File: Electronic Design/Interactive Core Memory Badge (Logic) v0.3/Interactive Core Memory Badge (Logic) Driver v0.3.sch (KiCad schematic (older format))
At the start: 64 parts, among them J1 SSW-116-22-F-S-VS‎, J2 SSW-116-22-F-S-VS‎, Q10 MMBT4401LT1G, Q11 MMBT4403LT1G, Q12 MMBT4401LT1G, Q13 MMBT4403LT1G, Q14 MMBT4401LT1G, Q15 MMBT4403LT1G, Q16 MMBT4401LT1G, Q17 MMBT4403LT1G, Q18 MMBT4401LT1G, Q19 MMBT4403LT1G, Q2 MMBT4403LT1G, Q20 MMBT4401LT1G, Q21 MMBT4403LT1G, Q22 MMBT4401LT1G, Q3 MMBT4401LT1G, Q4 MMBT4401LT1G, Q5 MMBT4403LT1G, Q6 MMBT4401LT1G, Q7 MMBT4403LT1G, Q8 MMBT4401LT1G, Q9 MMBT4403LT1G

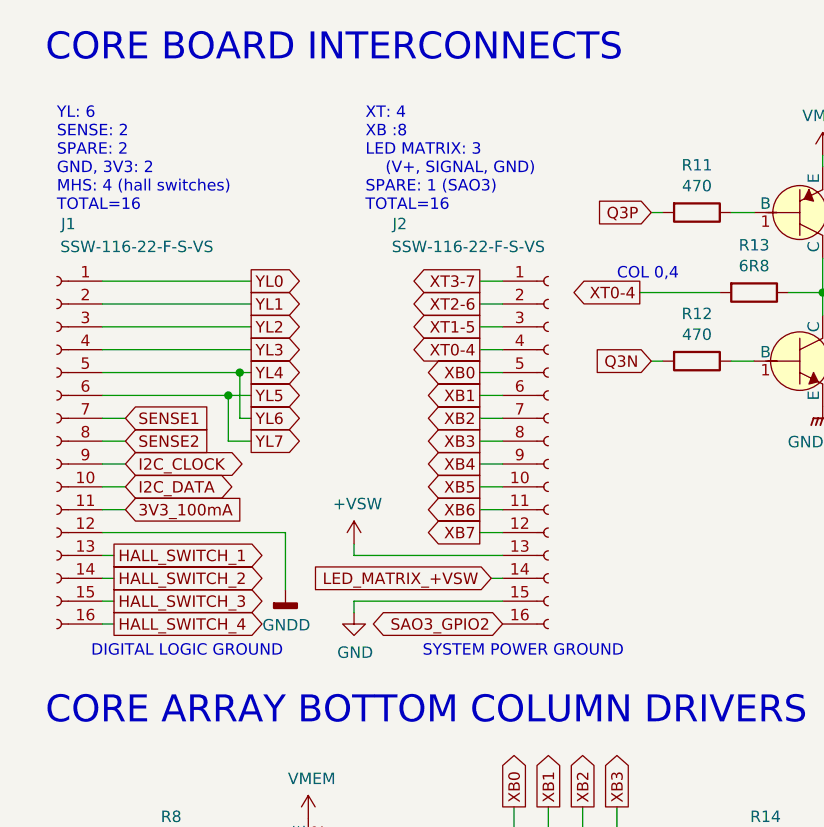
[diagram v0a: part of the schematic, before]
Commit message: Schematic review tweaks
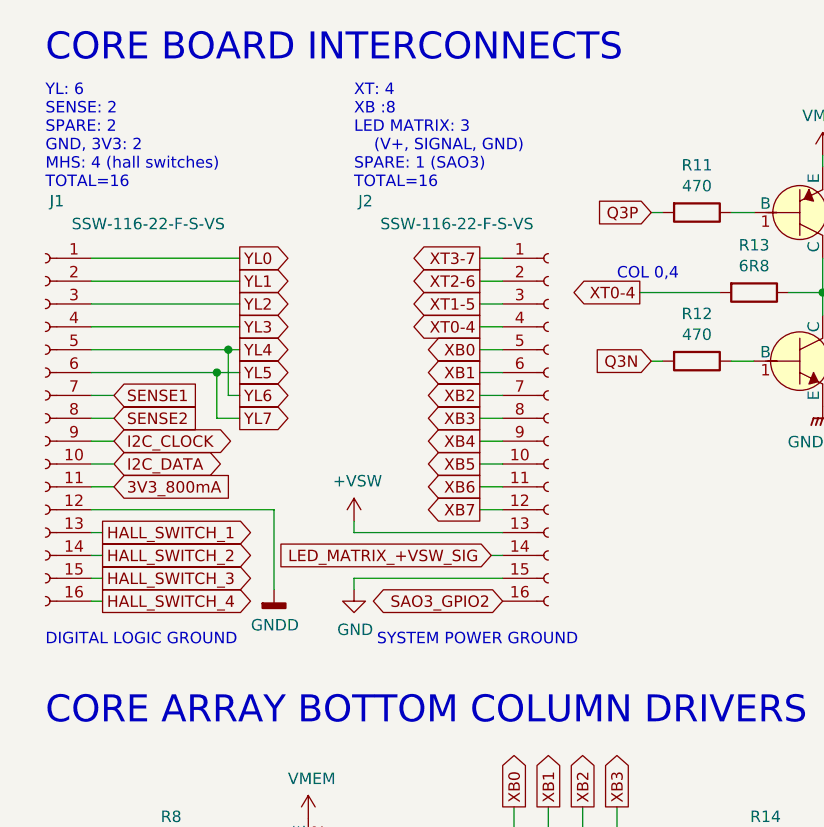
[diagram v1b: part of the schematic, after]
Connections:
- net 3V3_100mA is gone; now on net VMEM: J1.11 (Pin_11)
- net LED_MATRIX_+VSW renamed LED_MATRIX_+VSW_SIG
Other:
- moved on the sheet: J1, J2
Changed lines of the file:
@@
 Wire Wire Line
 	1200 4450 2400 4450
+Text GLabel 2450 2300 0    50   Output ~ 0
+XB3
+Text GLabel 2450 2200 0    50   Output ~ 0
+XB2
+Text GLabel 2450 2100 0    50   Output ~ 0
+XB1
+Text GLabel 2450 2000 0    50   Output ~ 0
+XB0
 Text GLabel 2450 2400 0    50   Output ~ 0
-XB3
-Text GLabel 2450 2300 0    50   Output ~ 0
-XB2
-Text GLabel 2450 2200 0    50   Output ~ 0
-XB1
-Text GLabel 2450 2100 0    50   Output ~ 0
-XB0
+XB4
 Text GLabel 2450 2500 0    50   Output ~ 0
-XB4
+XB5
 Text GLabel 2450 2600 0    50   Output ~ 0
-XB5
+XB6
 Text GLabel 2450 2700 0    50   Output ~ 0
-XB6
-Text GLabel 2450 2800 0    50   Output ~ 0
 XB7
-Text GLabel 2450 2000 0    50   Output ~ 0
+Text GLabel 2450 1900 0    50   Output ~ 0
 XT0-4
-Text GLabel 2450 1900 0    50   Output ~ 0
+Text GLabel 2450 1800 0    50   Output ~ 0
 XT1-5
-Text GLabel 2450 1800 0    50   Output ~ 0
+Text GLabel 2450 1700 0    50   Output ~ 0
 XT2-6
-Text GLabel 2450 1700 0    50   Output ~ 0
+Text GLabel 2450 1600 0    50   Output ~ 0
 XT3-7
 Wire Wire Line
+	2450 1600 2550 1600
+Wire Wire Line
 	2450 1700 2550 1700
 Wire Wire Line
@@
 Wire Wire Line
 	2450 1900 2550 1900
-Wire Wire Line
-	2450 2000 2550 2000
-Text GLabel 1450 1800 2    50   Output ~ 0
+Text GLabel 1400 1700 2    50   Output ~ 0
 YL1
-Text GLabel 1450 1700 2    50   Output ~ 0
+Text GLabel 1400 1600 2    50   Output ~ 0
 YL0
-Text GLabel 1450 1900 2    50   Output ~ 0
+Text GLabel 1400 1800 2    50   Output ~ 0
 YL2
-Text GLabel 1450 2000 2    50   Output ~ 0
+Text GLabel 1400 1900 2    50   Output ~ 0
 YL3
-Text GLabel 1450 2400 2    50   Output ~ 0
+Text GLabel 1400 2300 2    50   Output ~ 0
 YL7
 Wire Wire Line
-	1400 2100 1400 2300
-Wire Wire Line
-	1400 2300 1450 2300
-Wire Wire Line
-	1450 1700 800  1700
-Wire Wire Line
-	1450 2000 800  2000
-Wire Wire Line
-	1450 2100 1400 2100
-Wire Wire Line
-	1400 2100 800  2100
-Connection ~ 1400 2100
-Wire Wire Line
-	1350 2400 1450 2400
-Wire Wire Line
-	1350 2200 1350 2400
-Wire Wire Line
-	1450 2200 1350 2200
-Text Notes 600  1400 0    50   ~ 0
+	1350 2000 1350 2200
+Wire Wire Line
+	1350 2200 1400 2200
+Wire Wire Line
+	1400 1600 750  1600
+Wire Wire Line
+	1400 1900 750  1900
+Wire Wire Line
+	1400 2000 1350 2000
+Wire Wire Line
+	1350 2000 750  2000
+Connection ~ 1350 2000
+Wire Wire Line
+	1300 2300 1400 2300
+Wire Wire Line
+	1300 2100 1300 2300
+Wire Wire Line
+	1400 2100 1300 2100
+Text Notes 550  1300 0    50   ~ 0
 YL: 6\nSENSE: 2\nSPARE: 2\nGND, 3V3: 2\nMHS: 4 (hall switches)\nTOTAL=16
 Wire Wire Line
-	1350 2200 800  2200
-Connection ~ 1350 2200
-Wire Wire Line
-	2450 2800 2550 2800
+	1300 2100 750  2100
+Connection ~ 1300 2100
 Wire Wire Line
 	2450 2700 2550 2700
+Wire Wire Line
+	2450 2600 2550 2600
 $Comp
 L Connector:Conn_01x16_Female J2
 U 1 1 5E78B5ED
-P 2750 2400
-F 0 "J2" H 2100 3350 50  0000 C CNN
-F 1 "SSW-116-22-F-S-VS‎" H 2400 3250 50  0000 C CNN
-F 2 "Connector_PinHeader_2.54mm:PinHeader_1x16_P2.54mm_Vertical_SMD_and_TH_Pin1Left" H 2750 2400 50  0001 C CNN
-F 3 "~" H 2750 2400 50  0001 C CNN
-	1    2750 2400
+P 2750 2300
+F 0 "J2" H 1950 3250 50  0000 C CNN
+F 1 "SSW-116-22-F-S-VS‎" H 2350 3150 50  0000 C CNN
+F 2 "Connector_PinHeader_2.54mm:PinHeader_1x16_P2.54mm_Vertical_SMD_and_TH_Pin1Left" H 2750 2300 50  0001 C CNN
+F 3 "~" H 2750 2300 50  0001 C CNN
+	1    2750 2300
 	1    0    0    -1
 $EndComp
@@
 L Connector:Conn_01x16_Female J1
 U 1 1 5E78B5F3
-P 600 2400
-F 0 "J1" H 550 3350 50  0000 C CNN
-F 1 "SSW-116-22-F-S-VS‎" H 250 3250 50  0000 C CNN
-F 2 "Connector_PinHeader_2.54mm:PinHeader_1x16_P2.54mm_Vertical_SMD_and_TH_Pin1Left" H 600 2400 50  0001 C CNN
-F 3 "~" H 600 2400 50  0001 C CNN
-	1    600  2400
+P 550 2300
+F 0 "J1" H 500 3250 50  0000 C CNN
+F 1 "SSW-116-22-F-S-VS‎" H 100 3150 50  0000 C CNN
+F 2 "Connector_PinHeader_2.54mm:PinHeader_1x16_P2.54mm_Vertical_SMD_and_TH_Pin1Left" H 550 2300 50  0001 C CNN
+F 3 "~" H 550 2300 50  0001 C CNN
+	1    550  2300
 	-1   0    0    -1
 $EndComp
-Text Notes 1950 1400 0    50   ~ 0
+Text Notes 1900 1300 0    50   ~ 0
 XT: 4\nXB :8\nLED MATRIX: 3\n    (V+, SIGNAL, GND)\nSPARE: 1 (SAO3)\nTOTAL=16
 Wire Wire Line
-	2450 2400 2550 2400
-Wire Wire Line
-	2450 2600 2550 2600
-Text GLabel 900  2300 2    50   Input ~ 0
+	2450 2300 2550 2300
+Wire Wire Line
+	2450 2500 2550 2500
+Text GLabel 850  2200 2    50   Input ~ 0
 SENSE1
-Text GLabel 900  2400 2    50   Input ~ 0
+Text GLabel 850  2300 2    50   Input ~ 0
 SENSE2
 Wire Wire Line
-	900  2400 800  2400
-Text GLabel 2500 3000 0    50   Input ~ 0
-LED_MATRIX_+VSW
-Wire Wire Line
-	2500 3000 2550 3000
+	850  2300 750  2300
+Text GLabel 2500 2900 0    50   Input ~ 0
+LED_MATRIX_+VSW_SIG
+Wire Wire Line
+	2500 2900 2550 2900
 $Comp
 L power:GNDD #PWR0164
 U 1 1 5E78B651
-P 1600 3050
-F 0 "#PWR0164" H 1600 2800 50  0001 C CNN
-F 1 "GNDD" H 1604 2895 50  0000 C CNN
-F 2 "" H 1600 3050 50  0001 C CNN
-F 3 "" H 1600 3050 50  0001 C CNN
-	1    1600 3050
-	1    0    0    -1
-$EndComp
-Text GLabel 850  2900 2    50   Output ~ 0
+P 1550 3050
+F 0 "#PWR0164" H 1550 2800 50  0001 C CNN
+F 1 "GNDD" H 1554 2895 50  0000 C CNN
+F 2 "" H 1550 3050 50  0001 C CNN
+F 3 "" H 1550 3050 50  0001 C CNN
+	1    1550 3050
+	1    0    0    -1
+$EndComp
+Text GLabel 800  2800 2    50   Output ~ 0
 HALL_SWITCH_1
-Text GLabel 850  3000 2    50   Output ~ 0
+Text GLabel 800  2900 2    50   Output ~ 0
 HALL_SWITCH_2
-Text GLabel 850  3100 2    50   Output ~ 0
+Text GLabel 800  3000 2    50   Output ~ 0
 HALL_SWITCH_3
-Text GLabel 850  3200 2    50   Output ~ 0
+Text GLabel 800  3100 2    50   Output ~ 0
 HALL_SWITCH_4
 Wire Wire Line
-	1600 2800 1600 3050
-Wire Wire Line
-	800  2700 900  2700
-Wire Wire Line
-	800  2800 1600 2800
-Wire Wire Line
-	850  3000 800  3000
-Wire Wire Line
-	850  3200 800  3200
+	1550 2700 1550 3050
+Wire Wire Line
+	750  2600 850  2600
+Wire Wire Line
+	750  2700 1550 2700
+Wire Wire Line
+	800  2900 750  2900
+Wire Wire Line
+	800  3100 750  3100
+Wire Wire Line
+	2550 2000 2450 2000
 Wire Wire Line
 	2550 2100 2450 2100
@@
 	2550 2200 2450 2200
 Wire Wire Line
-	2550 2300 2450 2300
-Wire Wire Line
-	2550 2500 2450 2500
-Wire Wire Line
-	2550 3100 1900 3100
-Text Notes 750  3350 0    50   ~ 0
+	2550 2400 2450 2400
+Wire Wire Line
+	2550 3000 1900 3000
+Text Notes 550  3300 0    50   ~ 0
 DIGITAL LOGIC GROUND
 Text Notes 4200 7750 0    50   ~ 0
@@
 L power:GND #PWR?
 U 1 1 5E79F49F
-P 1900 3150
+P 1900 3050
 AR Path="/5D254AE8/5E79F49F" Ref="#PWR?"  Part="1"
 AR Path="/5E79F49F" Ref="#PWR?"  Part="1"
 AR Path="/5E755AC8/5E79F49F" Ref="#PWR0165"  Part="1"
-F 0 "#PWR0165" H 1900 2900 50  0001 C CNN
-F 1 "GND" H 1905 2975 50  0000 C CNN
-F 2 "" H 1900 3150 50  0001 C CNN
-F 3 "" H 1900 3150 50  0001 C CNN
-	1    1900 3150
-	1    0    0    -1
-$EndComp
-Text GLabel 900  2700 2    50   Input ~ 0
-3V3_100mA
-Wire Wire Line
-	800  1800 1450 1800
-Wire Wire Line
-	800  1900 1450 1900
-Wire Wire Line
-	800  2300 900  2300
-Wire Wire Line
-	800  2900 850  2900
-Wire Wire Line
-	800  3100 850  3100
-Text Notes 2200 3350 0    50   ~ 0
+F 0 "#PWR0165" H 1900 2800 50  0001 C CNN
+F 1 "GND" H 1905 2875 50  0000 C CNN
+F 2 "" H 1900 3050 50  0001 C CNN
+F 3 "" H 1900 3050 50  0001 C CNN
+	1    1900 3050
+	1    0    0    -1
+$EndComp
+Text GLabel 850  2600 2    50   Input ~ 0
+3V3_800mA
+Wire Wire Line
+	750  1700 1400 1700
+Wire Wire Line
+	750  1800 1400 1800
+Wire Wire Line
+	750  2200 850  2200
+Wire Wire Line
+	750  2800 800  2800
+Wire Wire Line
+	750  3000 800  3000
+Text Notes 2000 3300 0    50   ~ 0
 SYSTEM POWER GROUND
 Text Notes 550  750  0    118  ~ 0
@@
 L power:+VSW #PWR0122
 U 1 1 5E76A192
-P 1900 2850
-F 0 "#PWR0122" H 1900 2700 50  0001 C CNN
-F 1 "+VSW" H 1915 3025 50  0000 C CNN
-F 2 "" H 1900 2850 50  0001 C CNN
-F 3 "" H 1900 2850 50  0001 C CNN
-	1    1900 2850
-	1    0    0    -1
-$EndComp
-Wire Wire Line
-	1900 2900 1900 2850
-Wire Wire Line
-	1900 2900 2550 2900
+P 1900 2750
+F 0 "#PWR0122" H 1900 2600 50  0001 C CNN
+F 1 "+VSW" H 1915 2925 50  0000 C CNN
+F 2 "" H 1900 2750 50  0001 C CNN
+F 3 "" H 1900 2750 50  0001 C CNN
+	1    1900 2750
+	1    0    0    -1
+$EndComp
+Wire Wire Line
+	1900 2800 1900 2750
+Wire Wire Line
+	1900 2800 2550 2800
 Wire Wire Line
 	1450 7100 1900 7100
@@
 Wire Wire Line
 	1250 7400 1250 7500
-Text GLabel 900  2500 2    50   BiDi ~ 0
+Text GLabel 850  2400 2    50   BiDi ~ 0
 I2C_CLOCK
-Text GLabel 900  2600 2    50   BiDi ~ 0
+Text GLabel 850  2500 2    50   BiDi ~ 0
 I2C_DATA
-Text GLabel 1450 2300 2    50   Output ~ 0
+Text GLabel 1400 2200 2    50   Output ~ 0
 YL6
-Text GLabel 1450 2200 2    50   Output ~ 0
+Text GLabel 1400 2100 2    50   Output ~ 0
 YL5
-Text GLabel 1450 2100 2    50   Output ~ 0
+Text GLabel 1400 2000 2    50   Output ~ 0
 YL4
 Wire Wire Line
-	800  2500 900  2500
-Wire Wire Line
-	800  2600 900  2600
+	750  2400 850  2400
+Wire Wire Line
+	750  2500 850  2500
 Wire Wire Line
 	4200 6850 5300 6850
 Wire Wire Line
 	3800 7200 3900 7200
-Text GLabel 2550 3200 0    50   BiDi ~ 0
+Text GLabel 2550 3100 0    50   BiDi ~ 0
 SAO3_GPIO2
 Wire Wire Line
-	1900 3100 1900 3150
+	1900 3000 1900 3050
 $EndSCHEMATC
